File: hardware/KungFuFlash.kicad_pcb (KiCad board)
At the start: 2 copper layers, 60.6 x 62 mm, 40 parts, among them J1 USB Power, J2 USB_B_Micro, J4 SWD, Q1 BC817, SW1 Reset, SW2 Menu, SW3 Special, U1 C64-Exp-Port, U2 AMS1117-3.3, U3 STM32F405RGTx, Y1 8MHz

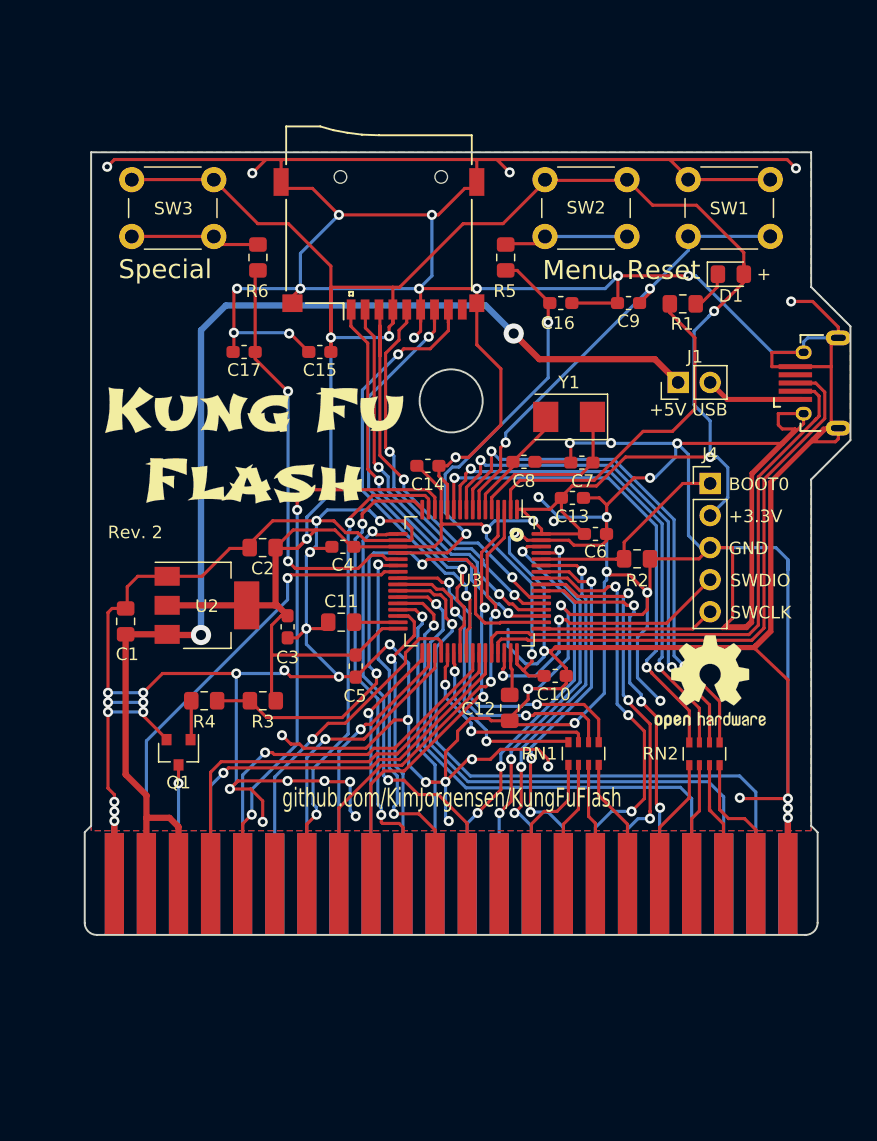
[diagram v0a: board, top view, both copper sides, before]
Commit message: Long board cart PCB layout.
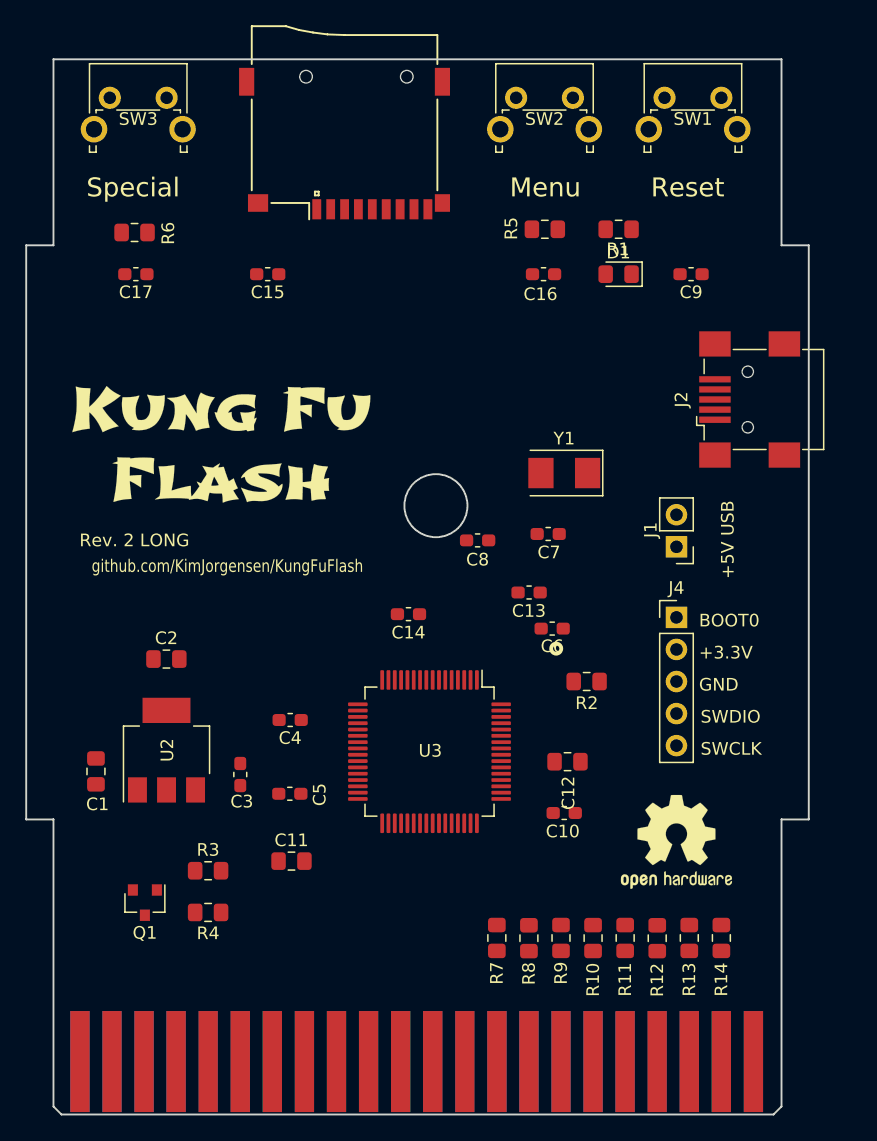
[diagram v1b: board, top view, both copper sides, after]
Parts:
- removed RN1, RN2: 100R, Resistor_SMD:R_Array_Convex_4x0603
- added R10: 100R, Resistor_SMD:R_0805_2012Metric_Pad1.15x1.40mm_HandSolder, F.Cu at (116.1, 130.4)
- added R11: 100R, Resistor_SMD:R_0805_2012Metric_Pad1.15x1.40mm_HandSolder, F.Cu at (118.7, 130.4)
- added R12: 100R, Resistor_SMD:R_0805_2012Metric_Pad1.15x1.40mm_HandSolder, F.Cu at (121.2, 130.4)
- added R13: 100R, Resistor_SMD:R_0805_2012Metric_Pad1.15x1.40mm_HandSolder, F.Cu at (123.8, 130.4)
- added R14: 100R, Resistor_SMD:R_0805_2012Metric_Pad1.15x1.40mm_HandSolder, F.Cu at (126.3, 130.4)
- added R7: 100R, Resistor_SMD:R_0805_2012Metric_Pad1.15x1.40mm_HandSolder, F.Cu at (108.5, 130.4)
- added R8: 100R, Resistor_SMD:R_0805_2012Metric_Pad1.15x1.40mm_HandSolder, F.Cu at (111.1, 130.4)
- added R9: 100R, Resistor_SMD:R_0805_2012Metric_Pad1.15x1.40mm_HandSolder, F.Cu at (113.6, 130.4)
- J2: value USB_B_Micro -> USB_B_Mini; footprint mod:Conn_USBmicro-B_ebay-side_TH -> Connector_USB:USB_Mini-B_Wuerth_65100516121_Horizontal
- SW1, SW2, SW3: footprint Button_Switch_THT:SW_PUSH_6mm_H8mm -> Button_Switch_THT:SW_Tactile_SPST_Angled_PTS645Vx83-2LFS
- moved C11 19.3 mm to (92.3, 124.3)
- moved R4 16.8 mm to (85.7, 128.4)
- moved U1 14.3 mm to (73.0, 144.1)
- moved C4 14.3 mm to (92.2, 113.2)
- moved R3 14.1 mm to (85.7, 125.1), turned to 0 degrees
- moved U3 13.9 mm to (103.2, 115.7)
- moved J1 13.0 mm to (122.7, 99.4), turned to 180 degrees
- moved REF** 12.9 mm to (122.7, 122.8)
- moved C3 12.3 mm to (88.2, 117.5)
- moved Q1 12.2 mm to (80.6, 127.6)
- moved C1 12.1 mm to (76.8, 117.2)
- moved U2 11.9 mm to (82.4, 115.5), turned to 90 degrees
- moved C14 11.8 mm to (101.5, 104.8)
- moved C2 11.7 mm to (82.4, 108.3), turned to 0 degrees
- moved C5 11.4 mm to (92.1, 119.0), turned to 0 degrees
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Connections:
- J2 pad 4: Net-(J2-Pad4) -> (no net)
- U1 pad 13: Net-(U1-Pad13) -> (no net)
- U1 pad 6: Net-(U1-Pad6) -> (no net)
- XS1 pad 9: Net-(XS1-Pad9) -> (no net)
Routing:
- net GND: track 751.1 -> 0.00 mm, vias 66 -> 0
- net +3V3: track 232.6 -> 0.00 mm, vias 8 -> 0
- net +5V: track 99.0 -> 0.00 mm, vias 2 -> 0
- net /A0: track 50.3 -> 0.00 mm, vias 1 -> 0
- net /A1: track 46.8 -> 0.00 mm, vias 1 -> 0
- net /USB_DP: track 45.1 -> 0.00 mm
- net /USB_DM: track 44.6 -> 0.00 mm
- net /R~W: track 44.5 -> 0.00 mm, vias 2 -> 0
- net /A2: track 43.6 -> 0.00 mm, vias 1 -> 0
- net /~RST_O: track 43.0 -> 0.00 mm, vias 2 -> 0
- net /D0: track 41.1 -> 0.00 mm, vias 2 -> 0
- net /D1: track 40.1 -> 0.00 mm, vias 2 -> 0
- net /D2: track 39.3 -> 0.00 mm, vias 2 -> 0
- net /D3: track 38.9 -> 0.00 mm, vias 2 -> 0
- net /~IO1: track 38.5 -> 0.00 mm, vias 2 -> 0
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- removed copper zone on B.Cu, net GND
- removed copper zone on F.Cu, net GND
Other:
- board size 60.6 x 62 mm -> 62 x 83.6 mm
- board text added: "Rev. 2 LONG"
- board text removed: "+"
- board text removed: "Rev. 2"
